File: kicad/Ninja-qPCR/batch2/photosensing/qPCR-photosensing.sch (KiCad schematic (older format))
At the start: 23 parts

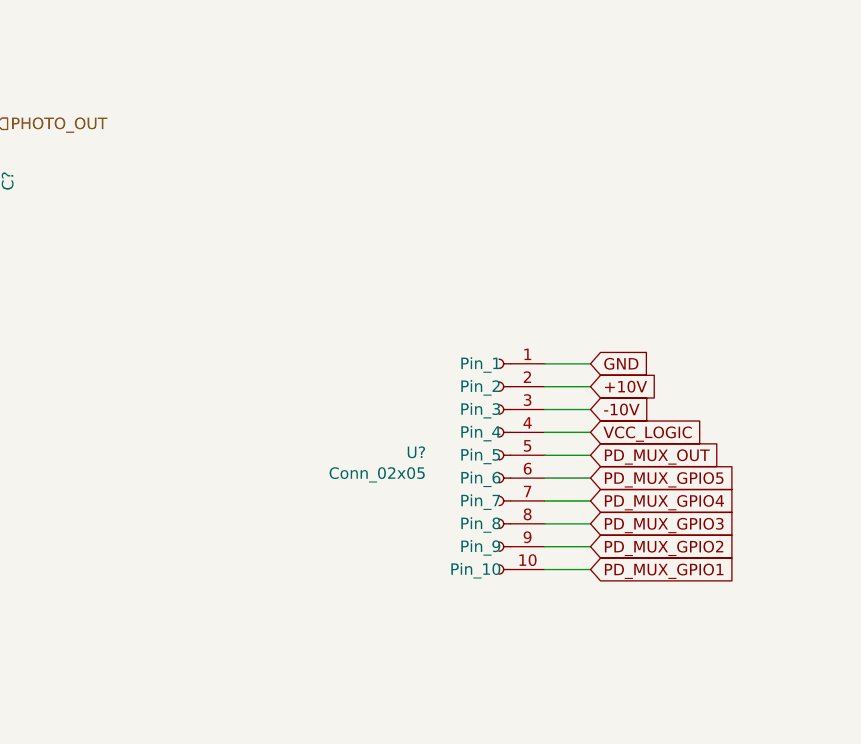
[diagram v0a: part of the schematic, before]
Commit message: sync
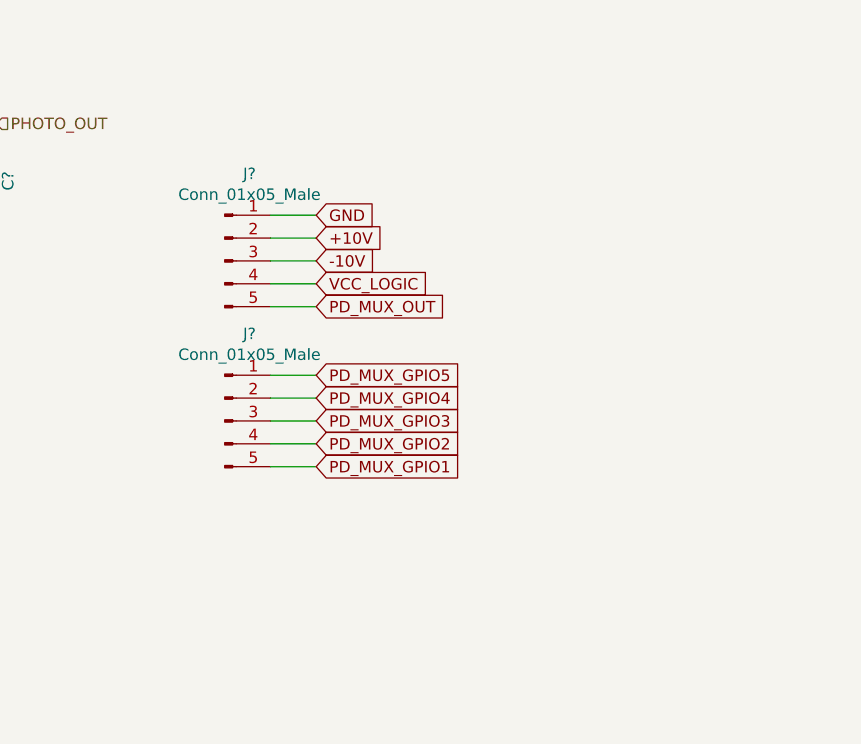
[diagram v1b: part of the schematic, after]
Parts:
- removed U?: Conn_02x05, symbol Ninja-qPCR:Conn_02x05
- added J? (x2): Conn_01x05_Male, symbol Connector:Conn_01x05_Male
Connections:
- net +10V: now also J?.2 (Pin_2)
- net -10V: now also J?.3 (Pin_3)
- net GND: now also J?.1 (Pin_1)
- net PD_MUX_GPIO1: now also J?.5 (Pin_5)
- net PD_MUX_GPIO2: now also J?.4 (Pin_4)
- net PD_MUX_GPIO3: now also J?.3 (Pin_3)
- net PD_MUX_GPIO4: now also J?.2 (Pin_2)
- net PD_MUX_GPIO5: now also J?.1 (Pin_1)
- net PD_MUX_OUT: now also J?.5 (Pin_5)
- net VCC_LOGIC: now also J?.4 (Pin_4)
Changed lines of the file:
@@
 Comment4 ""
 $EndDescr
-Text GLabel 10000 5300 2    50   Input ~ 0
-GND
-Text GLabel 10000 5400 2    50   Input ~ 0
+Text GLabel 8800 4650 2    50   Input ~ 0
+GND
+Text GLabel 8800 4750 2    50   Input ~ 0
 +10V
-Text GLabel 10000 5500 2    50   Input ~ 0
+Text GLabel 8800 4850 2    50   Input ~ 0
 -10V
 Wire Wire Line
-	9800 5300 10000 5300
-Wire Wire Line
-	10000 5400 9800 5400
-Wire Wire Line
-	9800 5500 10000 5500
-Wire Wire Line
-	10000 5600 9800 5600
-Wire Wire Line
-	9800 5700 10000 5700
-Wire Wire Line
-	10000 5800 9800 5800
-Wire Wire Line
-	9800 5900 10000 5900
-Wire Wire Line
-	10000 6000 9800 6000
-Wire Wire Line
-	9800 6100 10000 6100
-$Comp
-L Ninja-qPCR:Conn_02x05 U?
-U 1 1 5F51FB4B
-P 9600 5300
-F 0 "U?" H 9919 4911 50  0000 L CNN
-F 1 "Conn_02x05" H 9919 4820 50  0000 L CNN
-F 2 "" H 9400 5400 50  0001 C CNN
-F 3 "" H 9400 5400 50  0001 C CNN
-	1    9600 5300
-	-1   0    0    -1
-$EndComp
-Wire Wire Line
-	10000 6200 9800 6200
-Text GLabel 10000 5600 2    50   Input ~ 0
+	8600 4650 8800 4650
+Wire Wire Line
+	8800 4750 8600 4750
+Wire Wire Line
+	8600 4850 8800 4850
+Wire Wire Line
+	8800 4950 8600 4950
+Wire Wire Line
+	8600 5050 8800 5050
+Wire Wire Line
+	8800 5350 8600 5350
+Wire Wire Line
+	8600 5450 8800 5450
+Wire Wire Line
+	8800 5550 8600 5550
+Wire Wire Line
+	8600 5650 8800 5650
+Wire Wire Line
+	8800 5750 8600 5750
+Text GLabel 8800 4950 2    50   Input ~ 0
 VCC_LOGIC
-Text GLabel 10000 5700 2    50   Input ~ 0
+Text GLabel 8800 5050 2    50   Input ~ 0
 PD_MUX_OUT
-Text GLabel 10000 6200 2    50   Input ~ 0
+Text GLabel 8800 5750 2    50   Input ~ 0
 PD_MUX_GPIO1
-Text GLabel 10000 6100 2    50   Input ~ 0
+Text GLabel 8800 5650 2    50   Input ~ 0
 PD_MUX_GPIO2
-Text GLabel 10000 6000 2    50   Input ~ 0
+Text GLabel 8800 5550 2    50   Input ~ 0
 PD_MUX_GPIO3
-Text GLabel 10000 5900 2    50   Input ~ 0
+Text GLabel 8800 5450 2    50   Input ~ 0
 PD_MUX_GPIO4
-Text GLabel 10000 5800 2    50   Input ~ 0
+Text GLabel 8800 5350 2    50   Input ~ 0
 PD_MUX_GPIO5
 Text GLabel 1350 850  2    50   Input ~ 0
@@
 Text HLabel 7400 4250 2    50   Input ~ 0
 PHOTO_OUT
+$Comp
+L Connector:Conn_01x05_Male J?
+U 1 1 5F591AD7
+P 8400 4850
+F 0 "J?" H 8508 5231 50  0000 C CNN
+F 1 "Conn_01x05_Male" H 8508 5140 50  0000 C CNN
+F 2 "" H 8400 4850 50  0001 C CNN
+F 3 "~" H 8400 4850 50  0001 C CNN
+	1    8400 4850
+	1    0    0    -1
+$EndComp
+$Comp
+L Connector:Conn_01x05_Male J?
+U 1 1 5F59281D
+P 8400 5550
+F 0 "J?" H 8508 5931 50  0000 C CNN
+F 1 "Conn_01x05_Male" H 8508 5840 50  0000 C CNN
+F 2 "" H 8400 5550 50  0001 C CNN
+F 3 "~" H 8400 5550 50  0001 C CNN
+	1    8400 5550
+	1    0    0    -1
+$EndComp
 $EndSCHEMATC
